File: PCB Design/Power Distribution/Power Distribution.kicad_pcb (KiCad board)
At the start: 2 copper layers, 83.3 x 44.3 mm, 27 parts, among them J1 Barrel_Jack, J2 Barrel_Jack, J3 Barrel_Jack, J4 Barrel_Jack, J5 Barrel_Jack, J6 Switch Header Pin, J7 LED, Q1 2N7002, Q2 NCE30P30K, Q3 2N7002

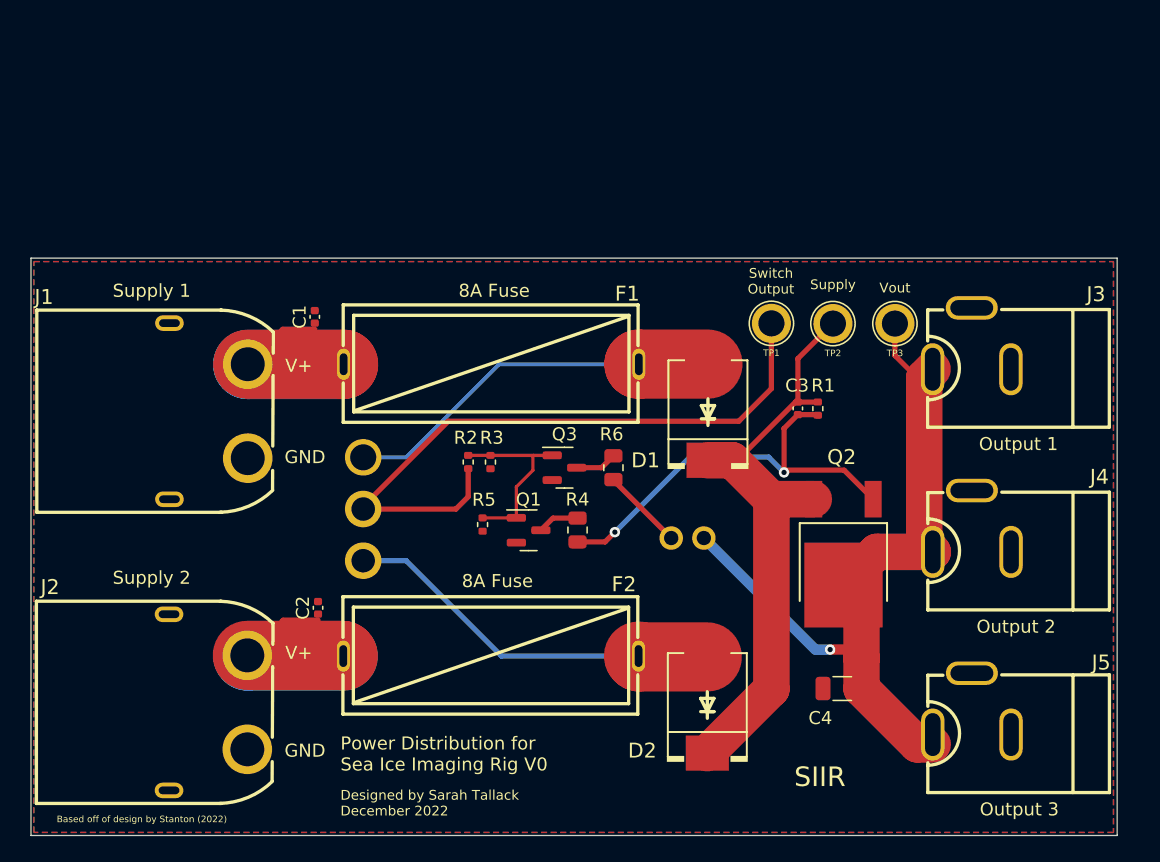
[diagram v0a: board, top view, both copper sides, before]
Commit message: $1
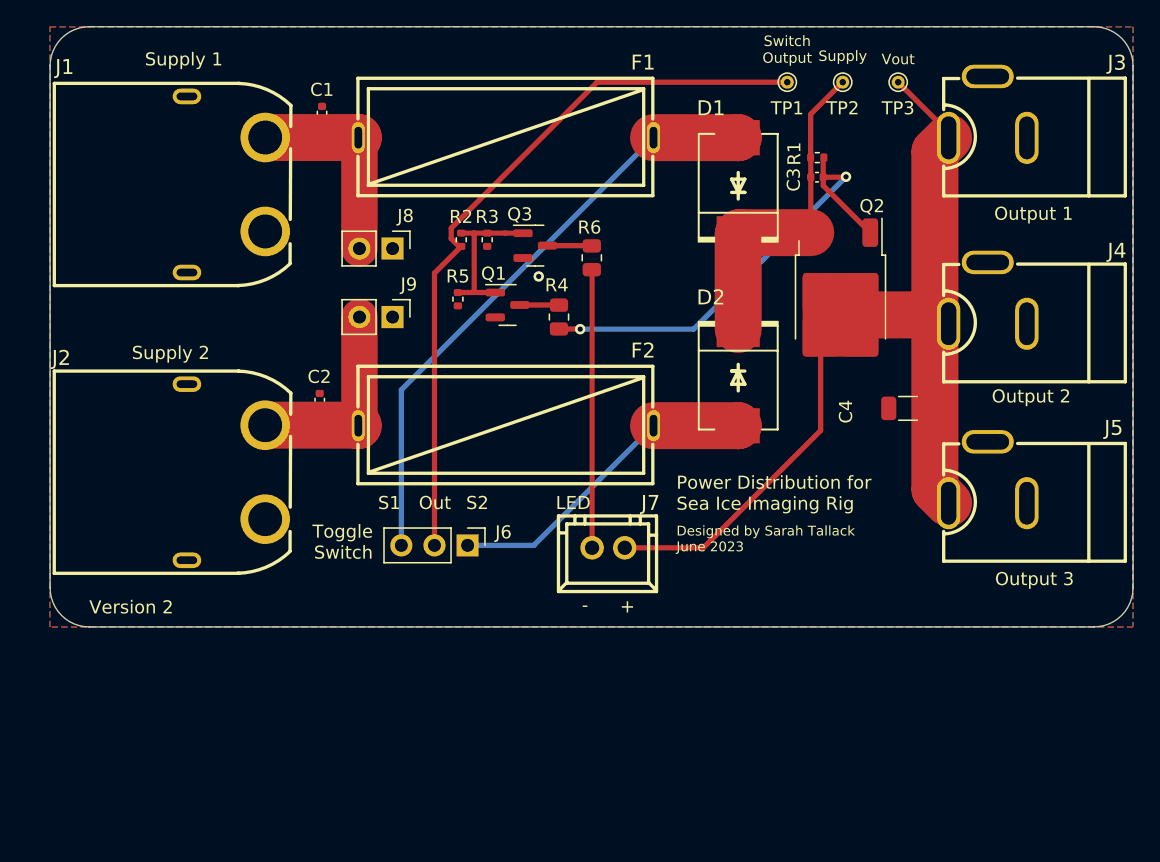
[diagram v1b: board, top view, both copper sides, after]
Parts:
- added J8: Conn_01x02_Pin, Connector_PinHeader_2.54mm:PinHeader_1x02_P2.54mm_Vertical, F.Cu at (212.2, 116.8)
- added J9: Conn_01x02_Pin, Connector_PinHeader_2.54mm:PinHeader_1x02_P2.54mm_Vertical, F.Cu at (212.2, 122.0)
- J6: footprint Footprints:3 Pin Male Header -> Connector_PinHeader_2.54mm:PinHeader_1x03_P2.54mm_Vertical; moved to F.Cu
- J7: moved to F.Cu
- Q2: footprint Footprints:NCE30P30K P channel MOSFET -> Package_TO_SOT_SMD:TO-252-2
- TP1, TP2, TP3: footprint TestPoint:TestPoint_Plated_Hole_D2.0mm -> TestPoint:TestPoint_THTPad_D1.0mm_Drill0.5mm
- moved D2 25.2 mm to (238.7, 126.6), turned to -90 degrees
- moved C4 22.1 mm to (251.8, 129.0)
- moved R1 19.2 mm to (244.8, 109.8), turned to 0 degrees
- moved Q2 18.7 mm to (246.6, 120.6)
- moved TP1 18.5 mm to (242.5, 104.0), turned to 90 degrees
- moved TP2 18.5 mm to (246.8, 104.0), turned to 90 degrees
- moved TP3 18.5 mm to (251.0, 104.0), turned to 90 degrees
- moved C3 17.8 mm to (244.8, 111.3), turned to 0 degrees
- moved J3 17.8 mm to (257.9, 105.9)
- moved J5 17.8 mm to (257.9, 133.9)
- moved F2 17.7 mm to (220.9, 130.3)
- moved J2 17.7 mm to (199.5, 133.9)
- moved J4 17.5 mm to (257.9, 120.2)
- moved D1 17.5 mm to (238.7, 111.9)
- moved J1 17.4 mm to (199.5, 111.8)
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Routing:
- net /Supply: track 48.2 -> 25.5 mm
- net /Mains: track 29.4 -> 45.7 mm
- net Net-(J7-Pin_2): track 6.27 -> 21.3 mm
- net /Vout: track 59.5 -> 68.9 mm, vias 1 -> 0
- net /Battery output: track 21.3 -> 15.5 mm
- net /AC/DC output: track 21.0 -> 15.7 mm
- net /Switch: track 50.8 -> 56.0 mm
- net /Battery: track 29.4 -> 24.5 mm
- net Net-(Q2-G): track 33.3 -> 35.9 mm
- net Net-(Q1-G): track 14.4 -> 12.2 mm
- net GND: vias 0 -> 1
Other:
- board size 83.3 x 44.3 mm -> 83 x 46 mm
- board text added: "Designed by Sarah Tallack June 2023"
- board text added: "LED"
- board text added: "Out"
- board text added: "S1"
- board text added: "S2"
- board text added: "Version 2"
- board text removed: "8A Fuse"
- board text removed: "Based off of design by Stanton (2022)"
- board text removed: "Designed by Sarah Tallack December 2022"
- board text removed: "GND"
- board text removed: "LED Indicator"
- board text removed: "Output"
- board text removed: "Power Distribution for Sea Ice Imaging Rig V0"
- board text removed: "SIIR"
- board text removed: "V+"
